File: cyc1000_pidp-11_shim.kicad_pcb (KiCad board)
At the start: 4 copper layers, 95 x 61 mm, 92 parts, among them J1 FTDI_FRIEND, J11 Raspberry_Hat, J12 RS232_PMOD, J13 USD_PMOD, J14 ETH_PMOD, J4 POWER, U1 CYC1000

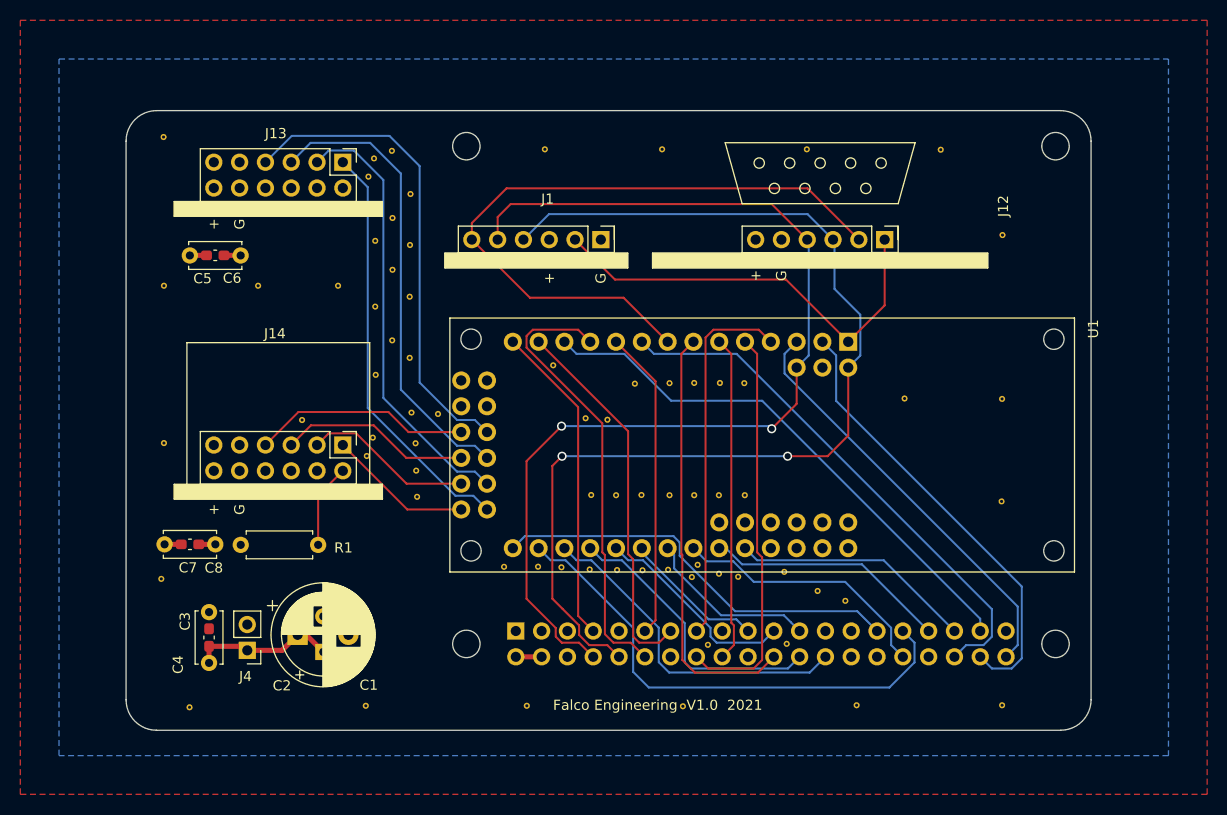
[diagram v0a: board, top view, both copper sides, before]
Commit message: Generate gerbers
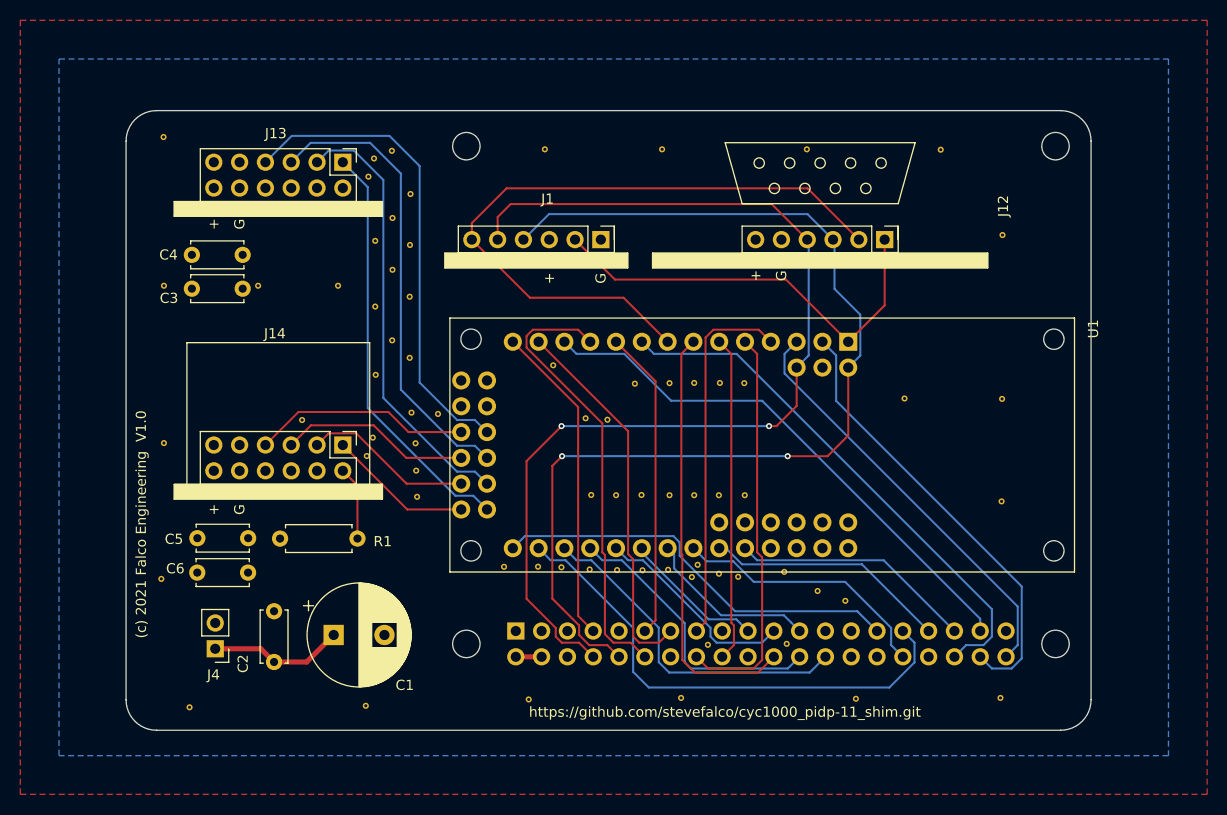
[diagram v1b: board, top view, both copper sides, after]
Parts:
- removed the C2 at (219.4, 142.3)
- removed the C3 at (208.2, 140.9)
- removed C7: 10u, Capacitor_SMD:C_0603_1608Metric_Pad1.08x0.95mm_HandSolder
- added C4: 0.1, Capacitor_THT:C_Disc_D5.0mm_W2.5mm_P5.00mm, F.Cu at (206.5, 103.2)
- C5: value 10u -> 0.1; footprint Capacitor_SMD:C_0603_1608Metric_Pad1.08x0.95mm_HandSolder -> Capacitor_THT:C_Disc_D5.0mm_W2.5mm_P5.00mm
- moved C5 27.9 mm to (207.0, 131.1)
- moved C2 6.40 mm to (214.6, 143.3)
- moved C6 4.25 mm to (207.0, 134.5)
- moved R1 3.92 mm to (222.8, 131.1)
- moved C1 3.55 mm to (220.4, 140.6)
- moved C3 3.28 mm to (206.5, 106.5)
- moved J4 3.16 mm to (208.8, 142.0)
- moved REF** 0.84 mm to (254.6, 146.8)
- moved REF** 0.74 mm to (286.1, 146.8)
- moved REF** 0.65 mm to (239.6, 147.0)
- moved REF** 0.64 mm to (271.9, 146.9)
- renumbered C4 to C2, C6 to C3, C8 to C6
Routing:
- net /VIN: track 71.7 -> 65.9 mm
- net /VCC33: track 3.28 -> 0.00 mm
- net GND: track 3.28 -> 0.00 mm
- net /INT: track 8.30 -> 7.27 mm
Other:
- net class Default: via_dia 0.9 -> 0.6; via_drill 0.6 -> 0.3
- rule trace_min: 0.1524 -> 0.127
- rule via_min_drill: 0.5 -> 0.254
- rule via_min_size: 0.8 -> 0.4572
- board text added: "(c) 2021 Falco Engineering V1.0"
- board text added: "THIS SHIM PCB IS VIEWED FROM THE TOP. IT PLUGS ONTO THE BACK OF THE PiDP-11 PCB. J11 must be installed on the bottom of this PCB in order to properly mate with the PiDP-11. The CYC1000 and all other parts are installed on the top of this PCB. All capacitors are optional. I personally prefer to include them. For C1, the square pad is the positive terminal and the round pad is the negative terminal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"
- board text added: "https://github.com/stevefalco/cyc1000_pidp-11_shim.git"
- board text removed: "Falco Engineering V1.0 2021"
- board text removed: "THIS SHIM PCB IS VIEWED FROM THE TOP. IT PLUGS ONTO THE BACK OF THE PiDP-11 PCB. J11 must be installed on the bottom of this PCB in order to properly mate with the PiDP-11. The CYC1000 and all other parts are installed on the top of this PCB. All capacitors are optional. I personally prefer to include them. For C1 / C2, the square pad is the positive terminal and the round pad is the negative ter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"
